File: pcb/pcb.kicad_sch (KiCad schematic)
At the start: 53 parts, among them J1 OLED, SW1 Rotary_Encoder_Switch, U1 Elite-C

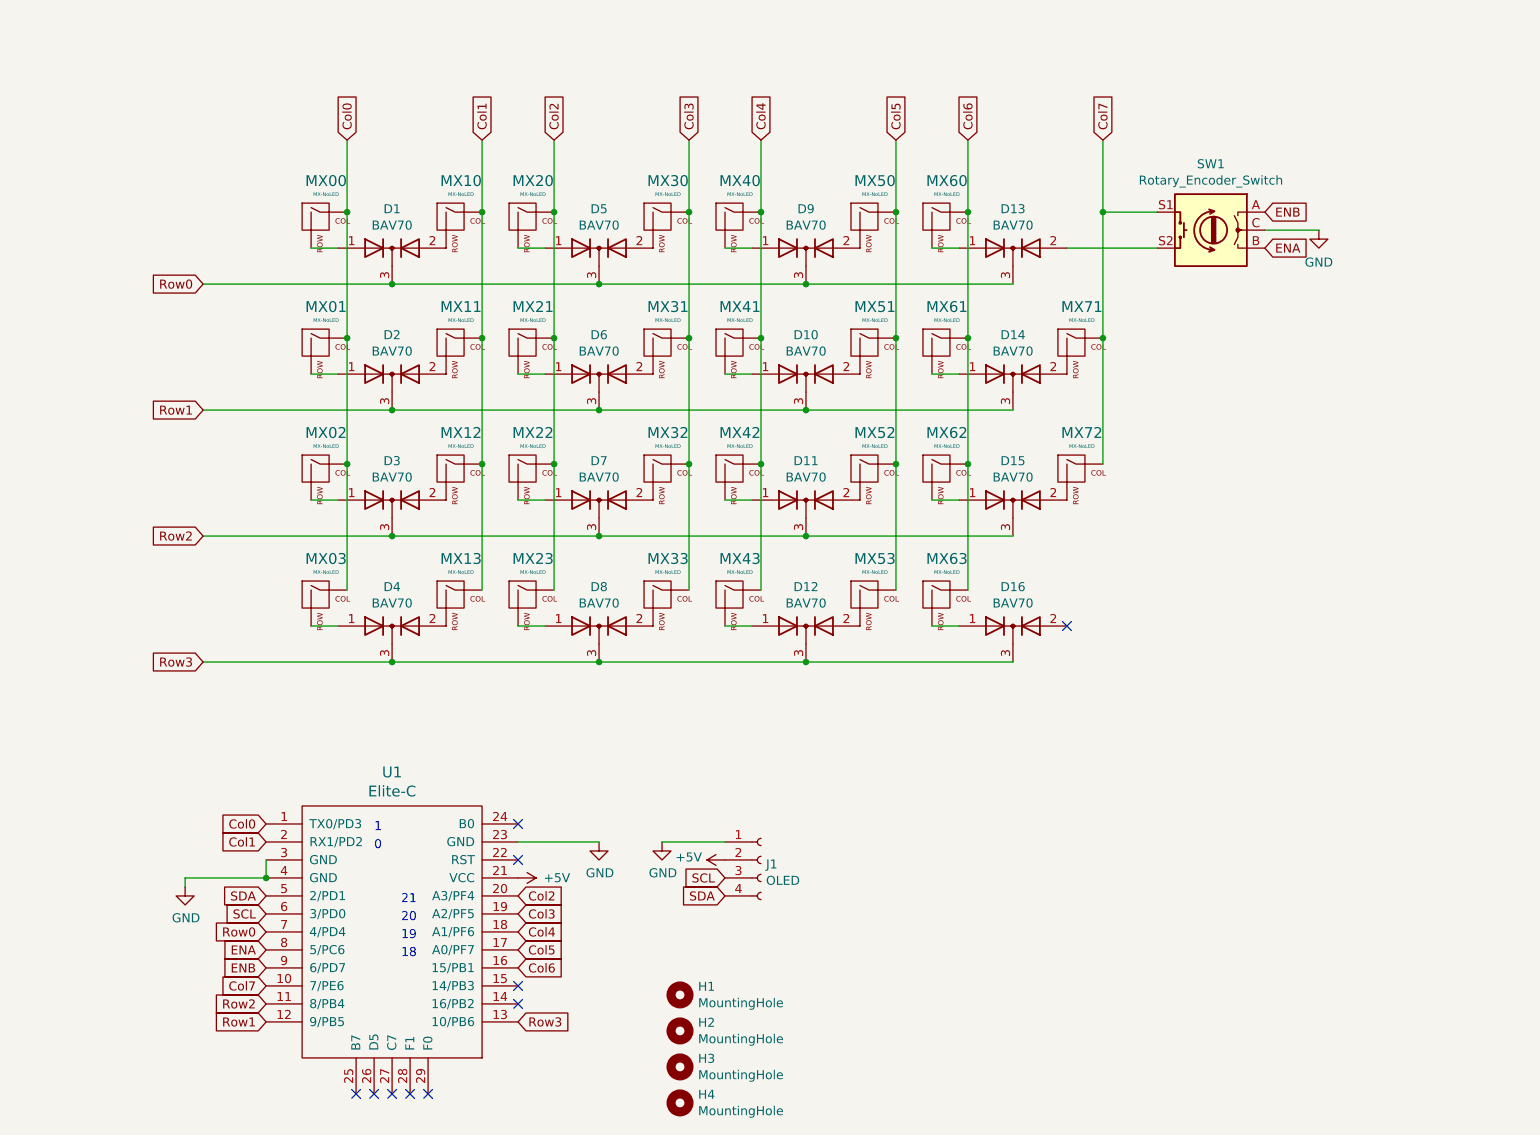
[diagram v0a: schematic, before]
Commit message: Added initial modified files.
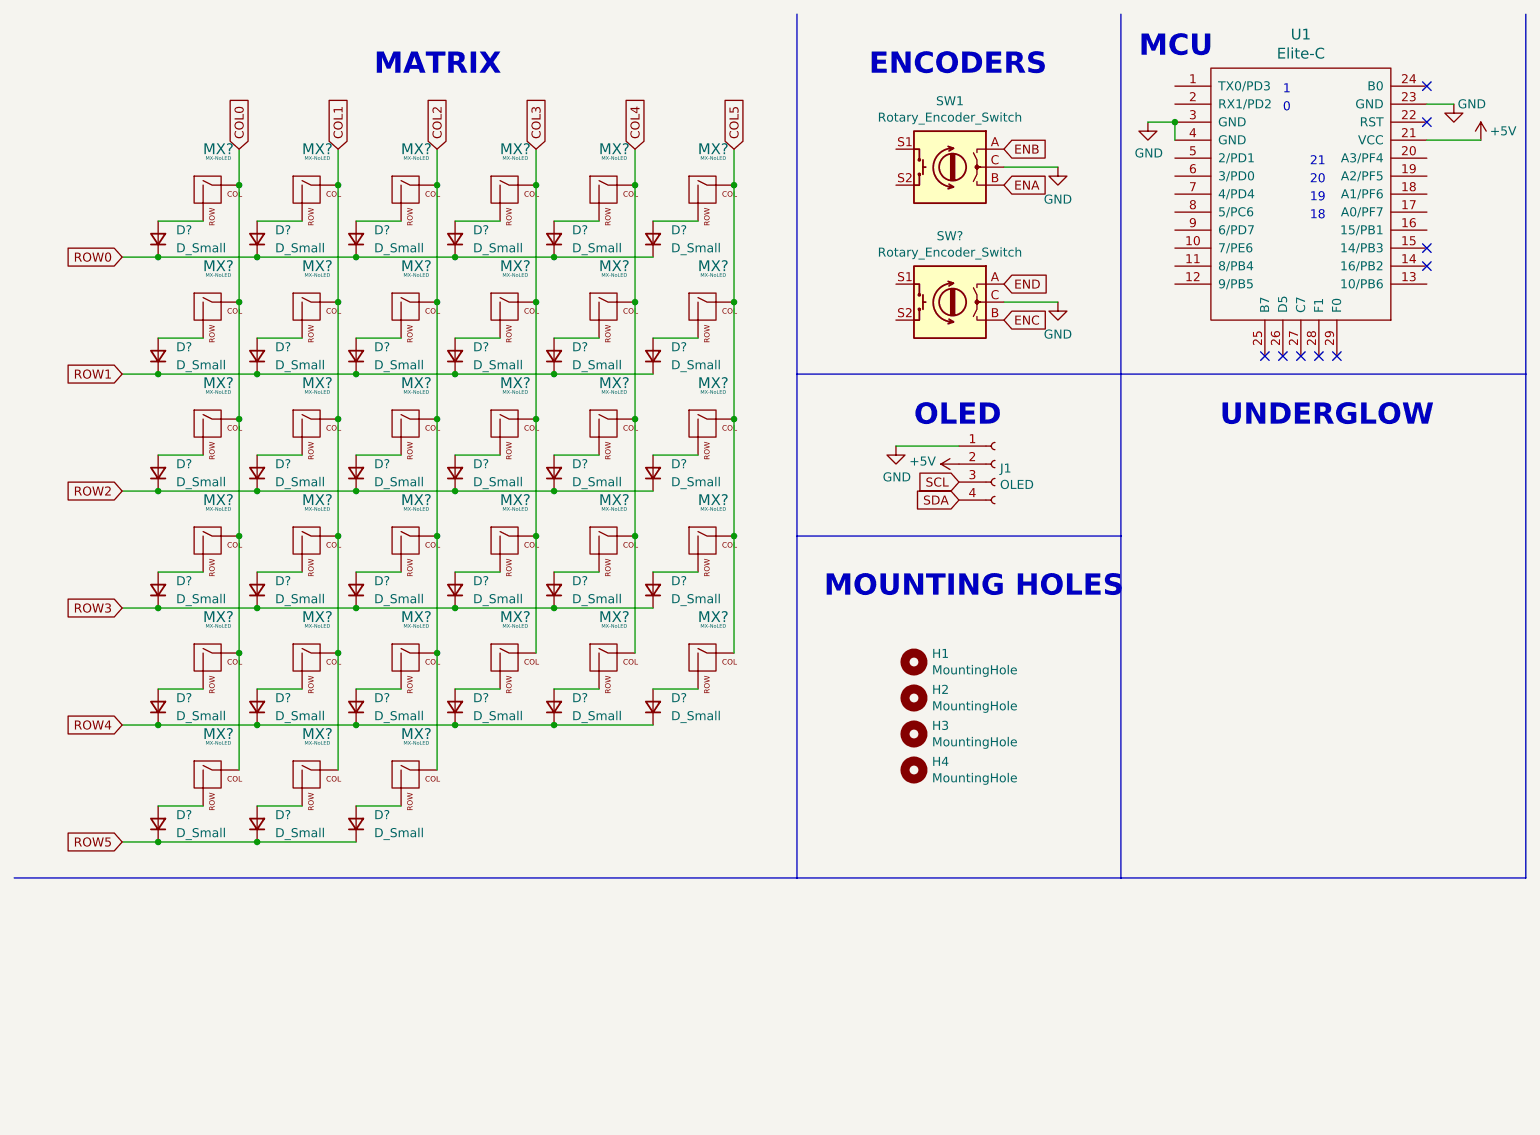
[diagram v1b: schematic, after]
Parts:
- removed D1, D10, D11, D12, D13, D14, D15, D16, D2, D3, D4, D5, D6, D7, D8, D9: BAV70, Keebio-Parts:SOT-23_Handsoldering, symbol Diode:BAV70
- removed MX00, MX10, MX11, MX12, MX13, MX20, MX21, MX22, MX23, MX30, MX31, MX32, MX33, MX40, MX41, MX42, MX43, MX50, MX51, MX52, MX53, MX60, MX61, MX62, MX63, MX71, MX72: MX-NoLED, MX_Only:MXOnly-1U-Hotswap, symbol MX_Alps_Hybrid:MX-NoLED
- removed MX01: MX-NoLED, MX_Only:MXOnly-1.5U-Hotswap, symbol MX_Alps_Hybrid:MX-NoLED
- removed MX02: MX-NoLED, MX_Only:MXOnly-1.75U-Hotswap, symbol MX_Alps_Hybrid:MX-NoLED
- removed MX03: MX-NoLED, MX_Only:MXOnly-2.25U-Hotswap, symbol MX_Alps_Hybrid:MX-NoLED
- added D? (x33): D_Small, symbol Device:D_Small
- added MX? (x33): MX-NoLED, symbol MX_Alps_Hybrid:MX-NoLED
- added SW?: Rotary_Encoder_Switch, Rotary_Encoder:RotaryEncoder_Alps_EC11E-Switch_Vertical_H20mm, symbol Device:Rotary_Encoder_Switch
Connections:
- net ENA: no longer U1.8 (5/PC6)
- net ENB: no longer U1.9 (6/PD7)
- net GND: now also SW?.C
- net SCL: no longer U1.6 (3/PD0)
- net SDA: no longer U1.5 (2/PD1)
- net Col0: no longer names the net of U1.1 (TX0/PD3)
- net Col1: no longer names the net of U1.2 (RX1/PD2)
- net Col2: no longer names the net of U1.20 (A3/PF4)
- net Col3: no longer names the net of U1.19 (A2/PF5)
- net Col4: no longer names the net of U1.18 (A1/PF6)
- net Col5: no longer names the net of U1.17 (A0/PF7)
- net Col6: no longer names the net of U1.16 (15/PB1)
- net Col7: no longer names the net of U1.10 (7/PE6)
- net Col7: no longer SW1.S1
- net Row0: no longer names the net of U1.7 (4/PD4)
- net Row1: no longer names the net of U1.12 (9/PB5)
- net Row2: no longer names the net of U1.11 (8/PB4)
- net Row3: no longer names the net of U1.13 (10/PB6)
- new net: D?.2 (A), MX?.2 (ROW) (x33)
- new net COL0: MX?.1 (COL), MX?.1 (COL), MX?.1 (COL), MX?.1 (COL), MX?.1 (COL), MX?.1 (COL)
- new net COL1: MX?.1 (COL), MX?.1 (COL), MX?.1 (COL), MX?.1 (COL), MX?.1 (COL), MX?.1 (COL)
- new net COL2: MX?.1 (COL), MX?.1 (COL), MX?.1 (COL), MX?.1 (COL), MX?.1 (COL), MX?.1 (COL)
- new net COL3: MX?.1 (COL), MX?.1 (COL), MX?.1 (COL), MX?.1 (COL), MX?.1 (COL)
- new net COL4: MX?.1 (COL), MX?.1 (COL), MX?.1 (COL), MX?.1 (COL), MX?.1 (COL)
- new net COL5: MX?.1 (COL), MX?.1 (COL), MX?.1 (COL), MX?.1 (COL), MX?.1 (COL)
- new net ENC: SW?.B
- new net END: SW?.A
- new net ROW0: D?.1 (K), D?.1 (K), D?.1 (K), D?.1 (K), D?.1 (K), D?.1 (K)
- new net ROW1: D?.1 (K), D?.1 (K), D?.1 (K), D?.1 (K), D?.1 (K), D?.1 (K)
- new net ROW2: D?.1 (K), D?.1 (K), D?.1 (K), D?.1 (K), D?.1 (K), D?.1 (K)
- new net ROW3: D?.1 (K), D?.1 (K), D?.1 (K), D?.1 (K), D?.1 (K), D?.1 (K)
- new net ROW4: D?.1 (K), D?.1 (K), D?.1 (K), D?.1 (K), D?.1 (K), D?.1 (K)
- new net ROW5: D?.1 (K), D?.1 (K), D?.1 (K)
- no-connect marks 10 -> 9
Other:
- note added: "ENCODERS"
- note added: "MATRIX"
- note added: "MCU"
- note added: "MOUNTING HOLES"
- note added: "OLED"
- note added: "UNDERGLOW"
- moved on the sheet: H1, H2, H3, H4, J1, SW1, U1
